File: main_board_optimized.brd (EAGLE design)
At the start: 91 x 66 mm, 49 parts, among them IC1 LT1168ACS8, IC2 LT1168ACS8, IC3 LT1168ACS8, IC4 317EMP, U1 TLC272IP, U2 TLC272IP, U3 TLC272IP

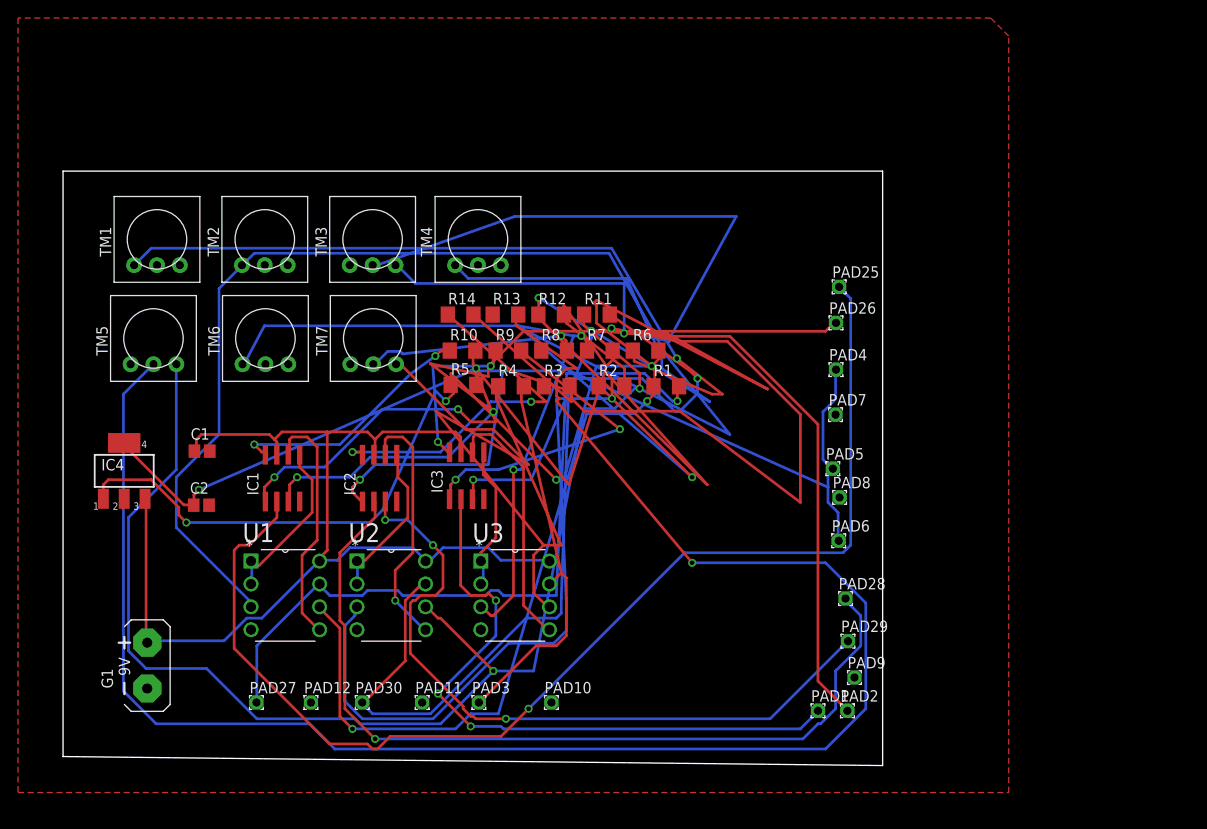
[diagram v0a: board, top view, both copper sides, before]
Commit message: Better layout
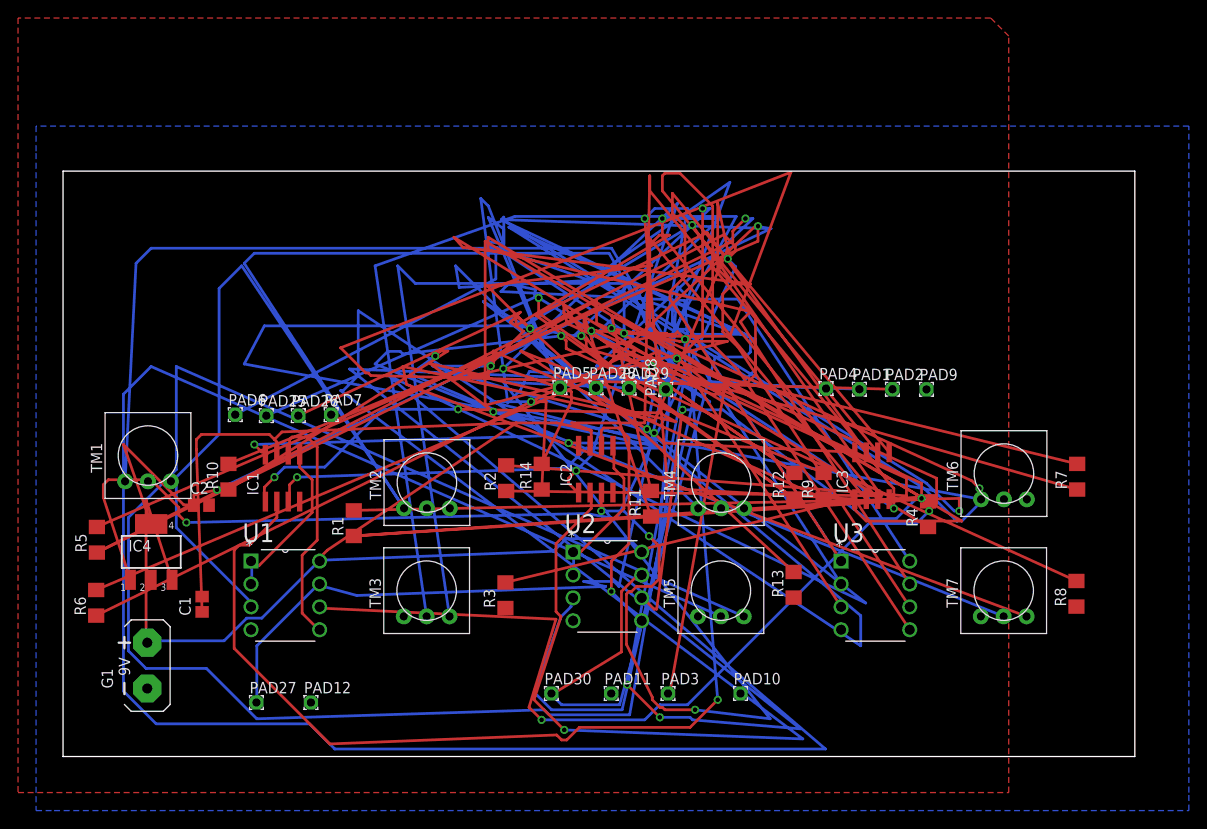
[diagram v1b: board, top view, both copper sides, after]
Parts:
- moved TM6 83.4 mm to (104.5, 31.4)
- moved TM7 75.4 mm to (104.4, 18.4)
- moved TM5 68.9 mm to (73.0, 18.4)
- moved PAD6 68.4 mm to (19.1, 38.0)
- moved R6 67.1 mm to (3.68, 17.1), turned to 90 degrees
- moved PAD25 65.2 mm to (22.6, 37.9)
- moved R8 64.0 mm to (112.5, 18.1), turned to 90 degrees
- moved PAD26 60.6 mm to (26.1, 37.9)
- moved PAD7 56.0 mm to (29.8, 38.0)
- moved R7 54.8 mm to (112.6, 31.1), turned to 90 degrees
- moved R4 48.4 mm to (96.0, 26.9), turned to 90 degrees
- moved IC3 45.0 mm to (89.8, 31.2)
- moved R5 44.2 mm to (3.76, 24.1), turned to 90 degrees
- moved R13 43.9 mm to (81.1, 19.1), turned to 90 degrees
- moved U3 40.0 mm to (94.0, 14.1)
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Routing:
- net VDD: track 164.7 -> 593.6 mm
- net N$6: track 94.3 -> 367.1 mm
- net N$27: track 196.0 -> 462.7 mm
- net N$2: track 159.7 -> 387.2 mm
- net VCC: track 120.0 -> 330.0 mm
- net N$25: track 180.2 -> 382.3 mm
- net N$8: track 79.9 -> 279.7 mm
- net N$11: track 77.8 -> 256.2 mm
- net N$24: track 143.0 -> 319.7 mm
- net N$1: track 83.9 -> 249.6 mm
- net N$32: track 96.3 -> 260.9 mm
- net N$18: track 72.1 -> 232.5 mm
- net N$5: track 128.8 -> 276.6 mm
- net N$9: track 16.2 -> 156.5 mm
- net N$13: track 23.6 -> 160.6 mm
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- added copper zone on layer 16, net N$33
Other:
- board size 91 x 66 mm -> 119 x 65 mm
